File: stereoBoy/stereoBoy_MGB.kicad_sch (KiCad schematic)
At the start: 0 parts

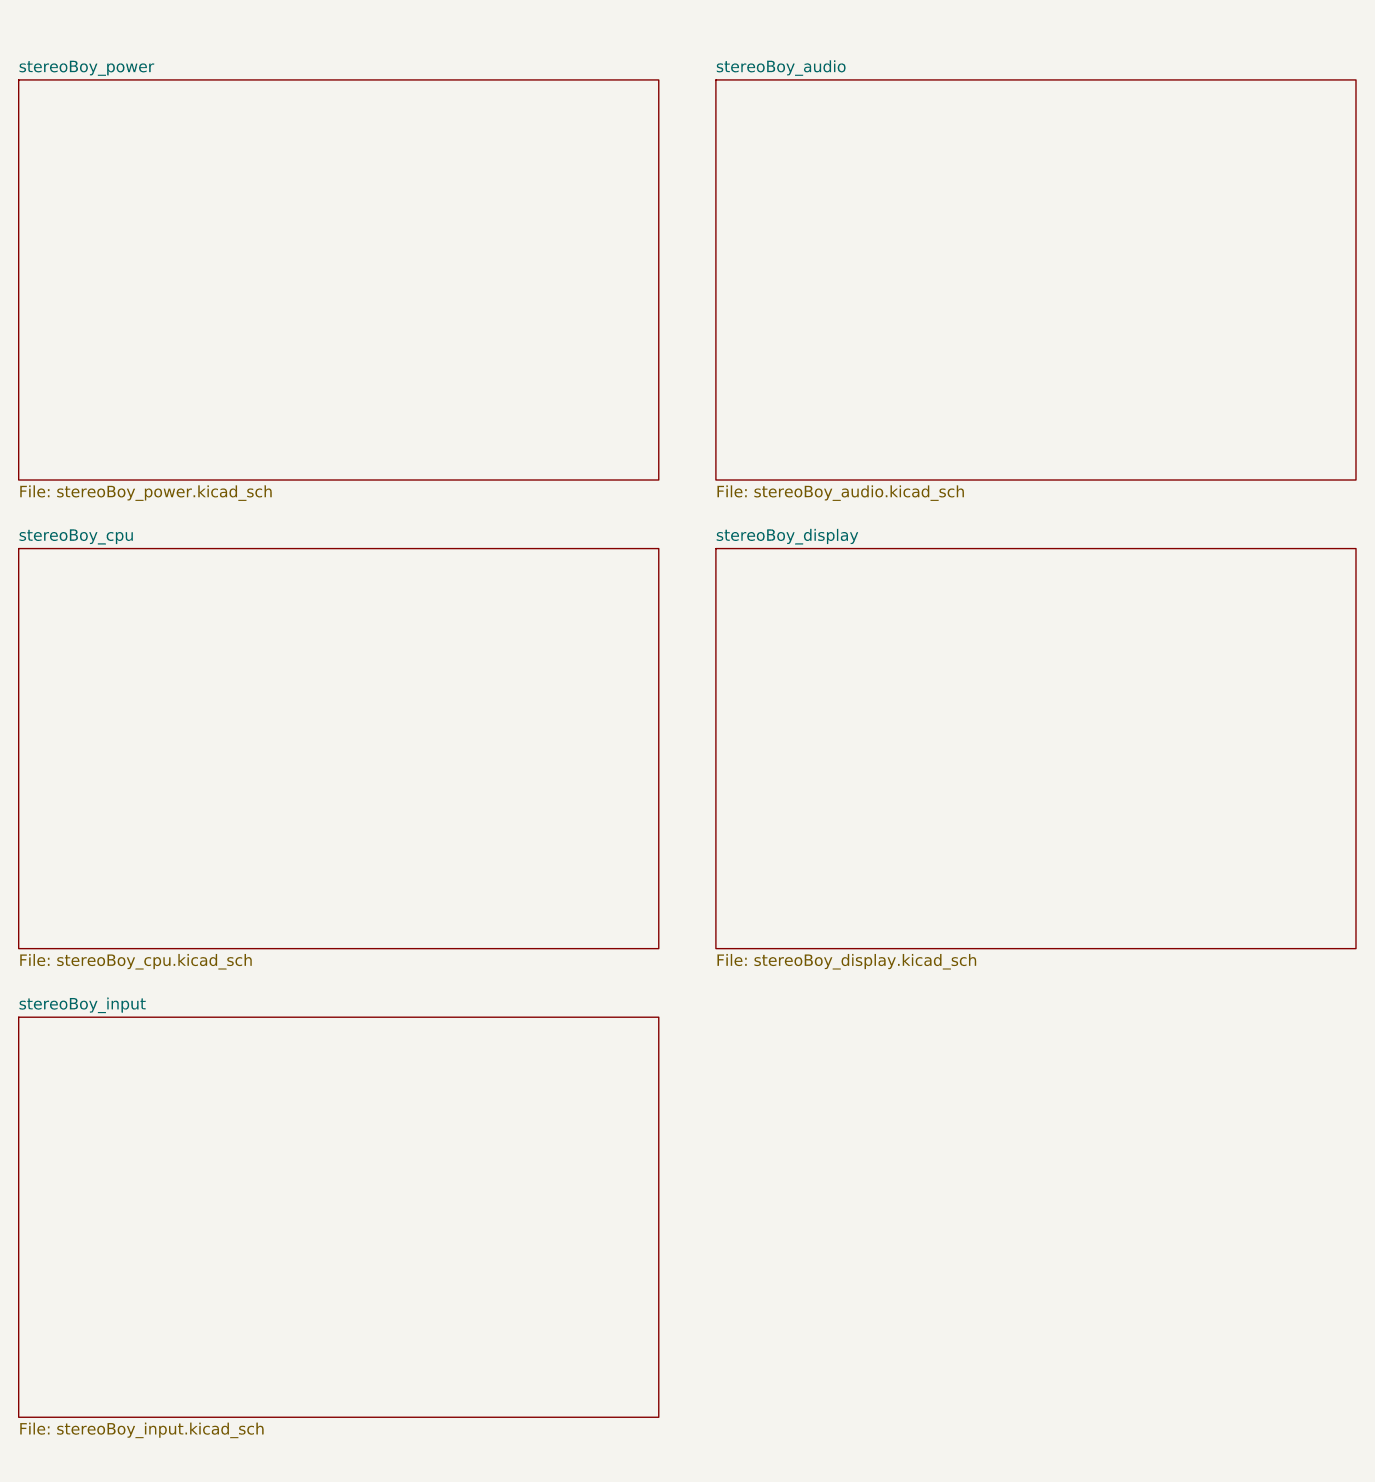
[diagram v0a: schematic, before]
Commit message: yuh
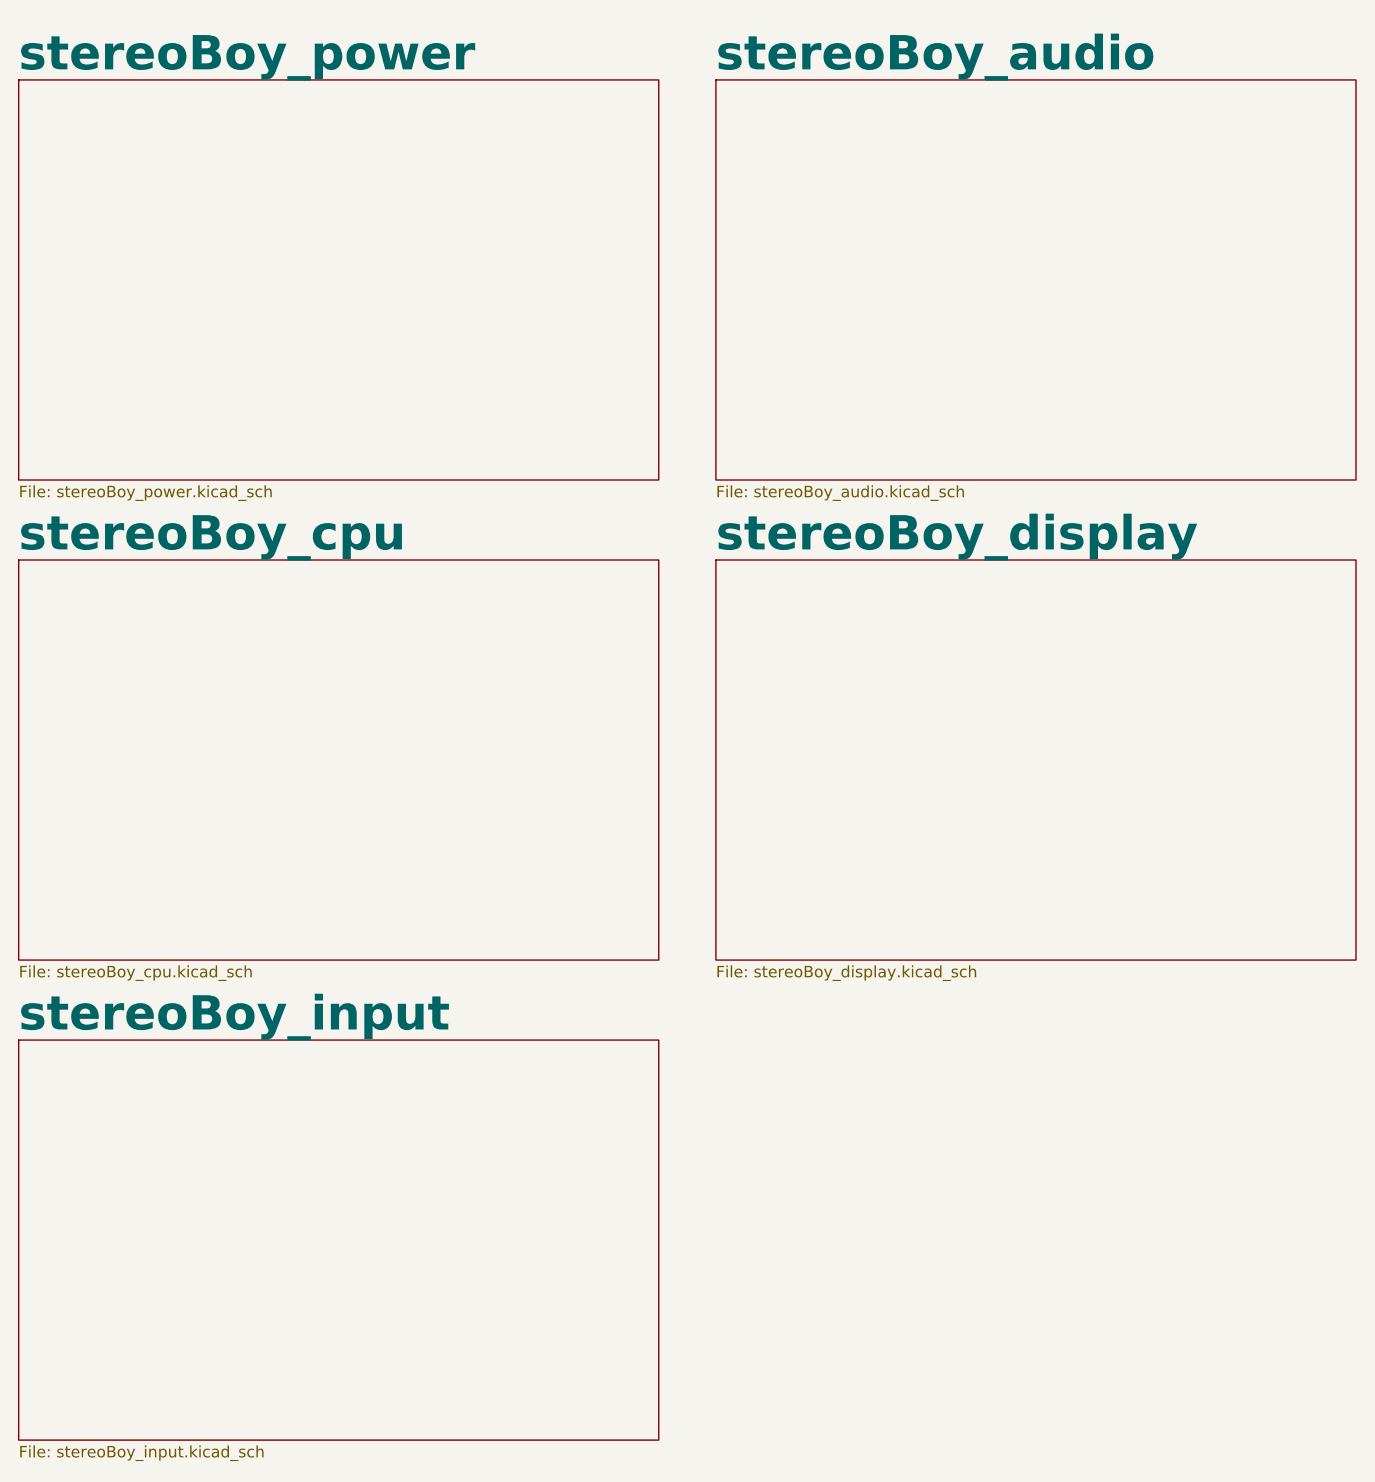
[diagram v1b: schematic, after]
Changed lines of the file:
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@@
 	(paper "User" 455.651 299.872)
 	(sheet
-		(at 119.38 83.82)
+		(at 119.38 85.09)
 		(size 71.12 44.45)
 		(exclude_from_sim no)
@@
 		)
 		(property "Sheetname" "stereoBoy_display"
-			(at 119.38 83.1084 0)
-			(effects
-				(font
-					(size 1.27 1.27)
+			(at 119.38 84.3784 0)
+			(effects
+				(font
+					(size 3.81 3.81)
+					(thickness 0.762)
+					(bold yes)
 				)
 				(justify left bottom)
@@
 		)
 		(property "Sheetfile" "stereoBoy_display.kicad_sch"
-			(at 119.38 128.8546 0)
+			(at 119.38 130.1246 0)
 			(effects
 				(font
@@
 			(effects
 				(font
-					(size 1.27 1.27)
+					(size 3.81 3.81)
+					(thickness 0.762)
+					(bold yes)
 				)
 				(justify left bottom)
@@
 	)
 	(sheet
-		(at 41.91 135.89)
+		(at 41.91 138.43)
 		(size 71.12 44.45)
 		(exclude_from_sim no)
@@
 		)
 		(property "Sheetname" "stereoBoy_input"
-			(at 41.91 135.1784 0)
-			(effects
-				(font
-					(size 1.27 1.27)
+			(at 41.91 137.7184 0)
+			(effects
+				(font
+					(size 3.81 3.81)
+					(thickness 0.762)
+					(bold yes)
 				)
 				(justify left bottom)
@@
 		)
 		(property "Sheetfile" "stereoBoy_input.kicad_sch"
-			(at 41.91 180.9246 0)
+			(at 41.91 183.4646 0)
 			(effects
 				(font
@@
 			(effects
 				(font
-					(size 1.27 1.27)
+					(size 3.81 3.81)
+					(thickness 0.762)
+					(bold yes)
 				)
 				(justify left bottom)
@@
 	)
 	(sheet
-		(at 41.91 83.82)
+		(at 41.91 85.09)
 		(size 71.12 44.45)
 		(exclude_from_sim no)
@@
 		)
 		(property "Sheetname" "stereoBoy_cpu"
-			(at 41.91 83.1084 0)
-			(effects
-				(font
-					(size 1.27 1.27)
+			(at 41.91 84.3784 0)
+			(effects
+				(font
+					(size 3.81 3.81)
+					(thickness 0.762)
+					(bold yes)
 				)
 				(justify left bottom)
@@
 		)
 		(property "Sheetfile" "stereoBoy_cpu.kicad_sch"
-			(at 41.91 128.8546 0)
-			(effects
-				(font
+			(at 41.91 130.1246 0)
+			(effects
+				(font
